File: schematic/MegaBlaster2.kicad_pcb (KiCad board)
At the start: 4 copper layers, 99 x 99 mm, 120 parts, among them J1 USB_B, J2 SWD, J3 Micro_SD_Card, J4 AudioJack3, SW2 SW_Push_Dual, SW3 SW_Push_Dual, SW4 SW_Push_Dual, SW5 SW_Push_Dual, SW6 SW_Push_Dual, SW7 SW_Push_Dual, SW8 YM_SELECTION, U1 ATSAMD51J19A-A, U10 TPA6111A2DR, U11 NE5532, U2 LM2733XMF, U3 LD1117S33TR_SOT223, U4 LD1117S50TR_SOT223, U5 W25Q32JVSS, U6 Si5351A-B-GT, U7 RAM_EXP, U8 YM2612, U9 SN76489, Y1 32.768KHz, Y2 25MHz

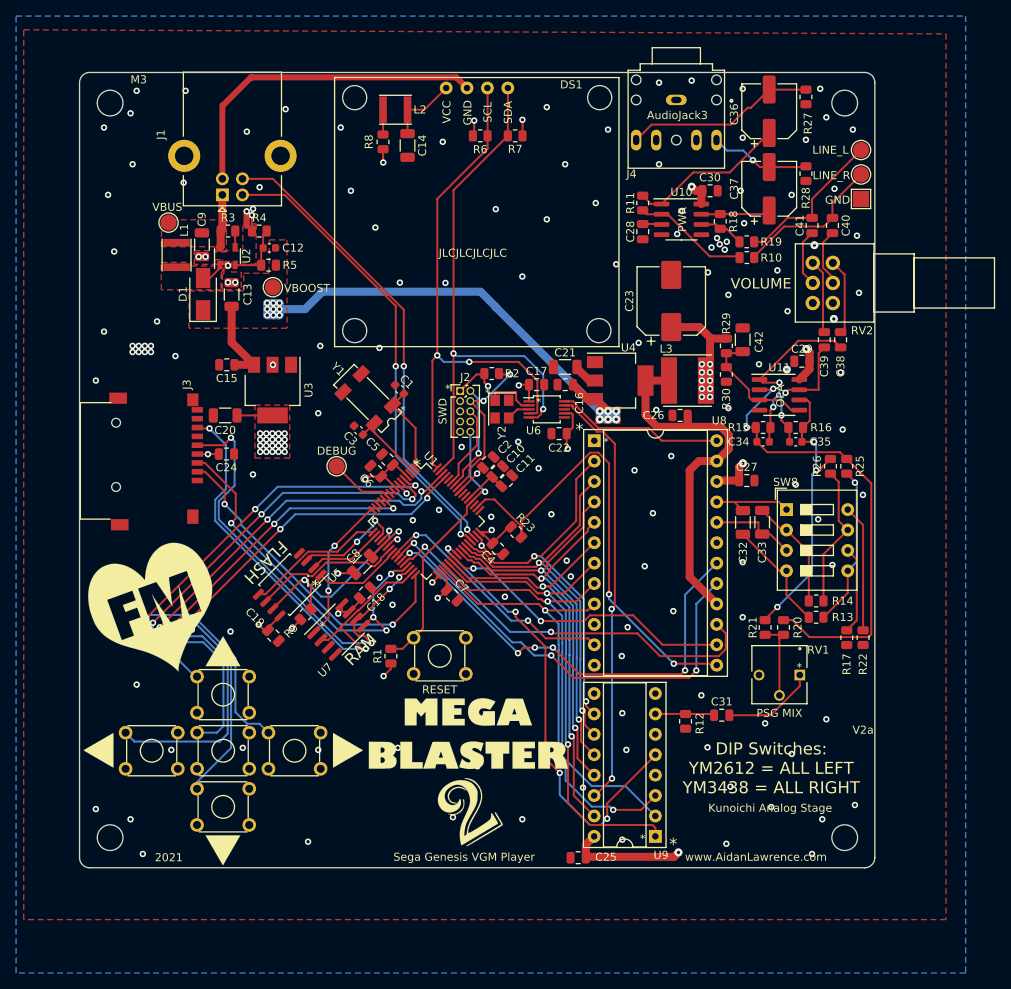
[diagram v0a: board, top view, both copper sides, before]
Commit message: schematic v1
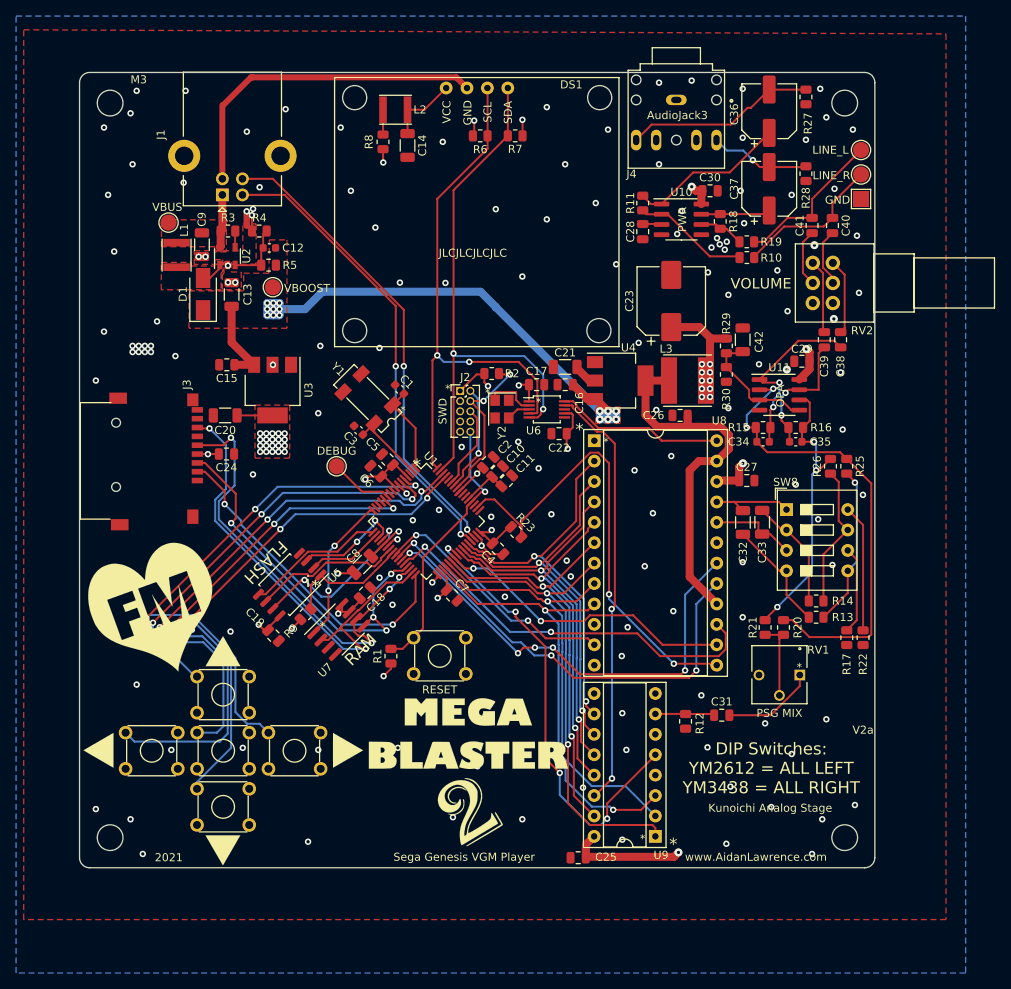
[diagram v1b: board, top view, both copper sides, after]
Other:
- net class Default removed
- net class THICC removed
